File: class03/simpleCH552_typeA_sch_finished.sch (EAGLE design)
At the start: 15 parts, among them U2 CH552G, X1 USBPCB

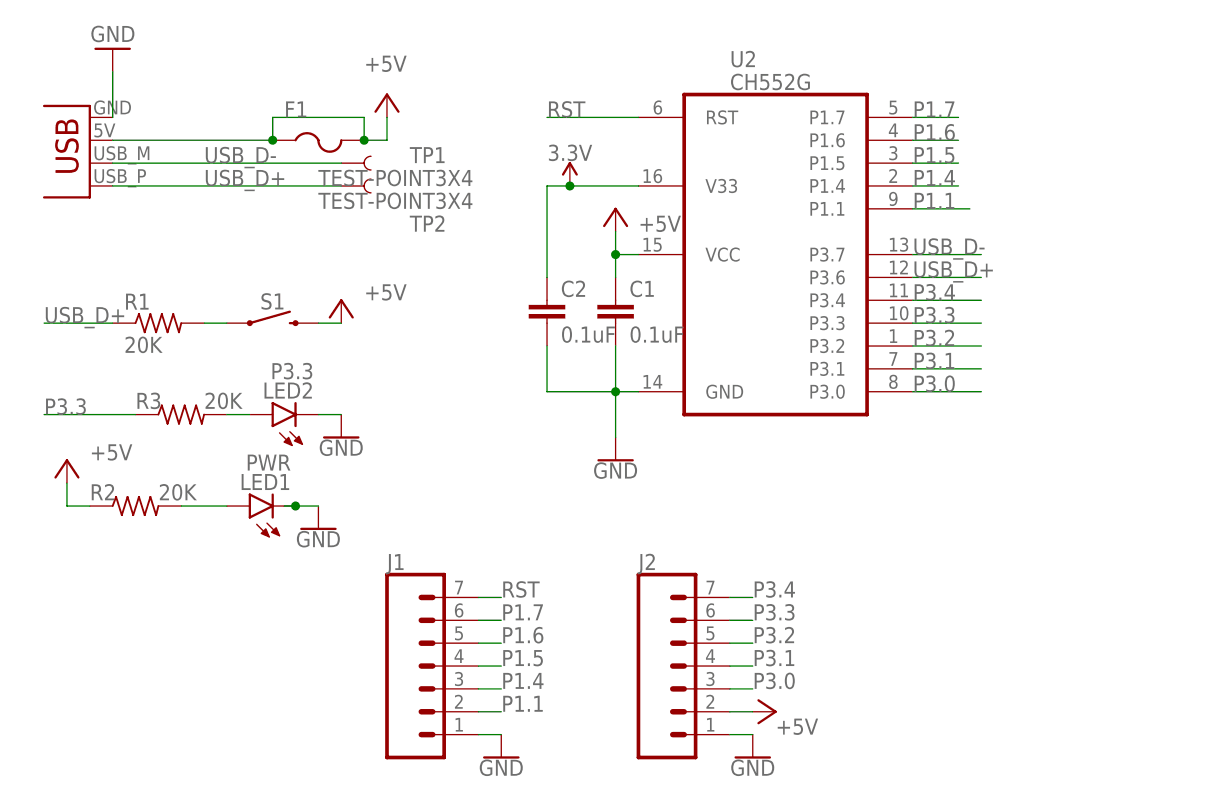
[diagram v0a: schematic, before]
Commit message: change sch finished
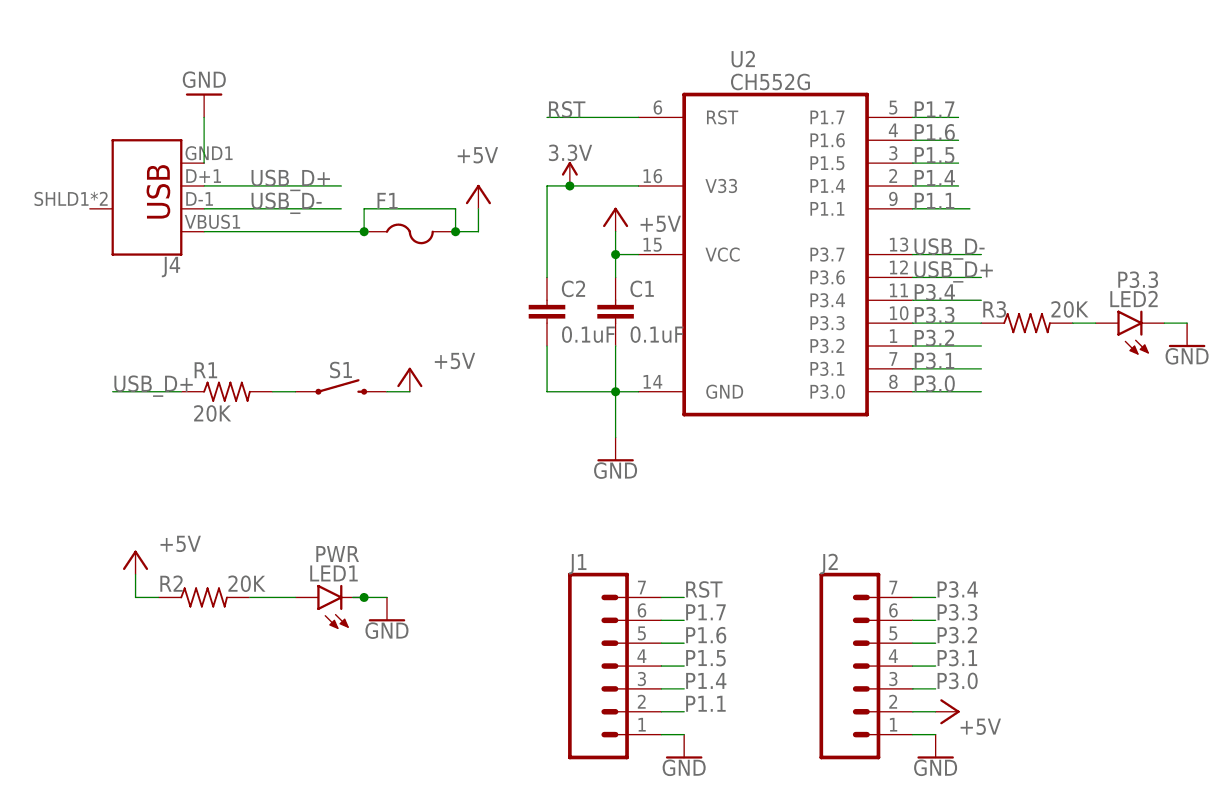
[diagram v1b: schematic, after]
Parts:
- removed TP1, TP2: TEST-POINT3X4, SparkFun-Connectors:TEST-POINT3X4
- removed X1: USBPCB, SparkFun:USBPCB
- added J4: USB_A_SMT_MALE, SparkFun-Connectors:USB_A_SMT_MALE
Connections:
- net +5V: now also J4.VBUS; no longer X1.VBUS
- net GND: now also J4.GND; no longer X1.GND
- net USB_D+: now also J4.D+; no longer TP2.1, X1.D+
- net USB_D-: now also J4.D-; no longer TP1.1, X1.D-
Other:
- moved on the sheet: F1, J1, J2, LED1, LED2, R1, R2, R3, S1
